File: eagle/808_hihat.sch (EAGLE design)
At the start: 127 parts, among them IC1 TL072P, IC2 TL072P, Q21* BC546, Q22* BC546, Q23* BC546, Q24* BC546, Q26* BC546, Q27* BC546, Q28* BC546, Q29* BC546, Q3* BC546, Q30* BC546, Q31* BC546, Q4* BC546, Q7* BC556, Q8* BC556, U4 4584N

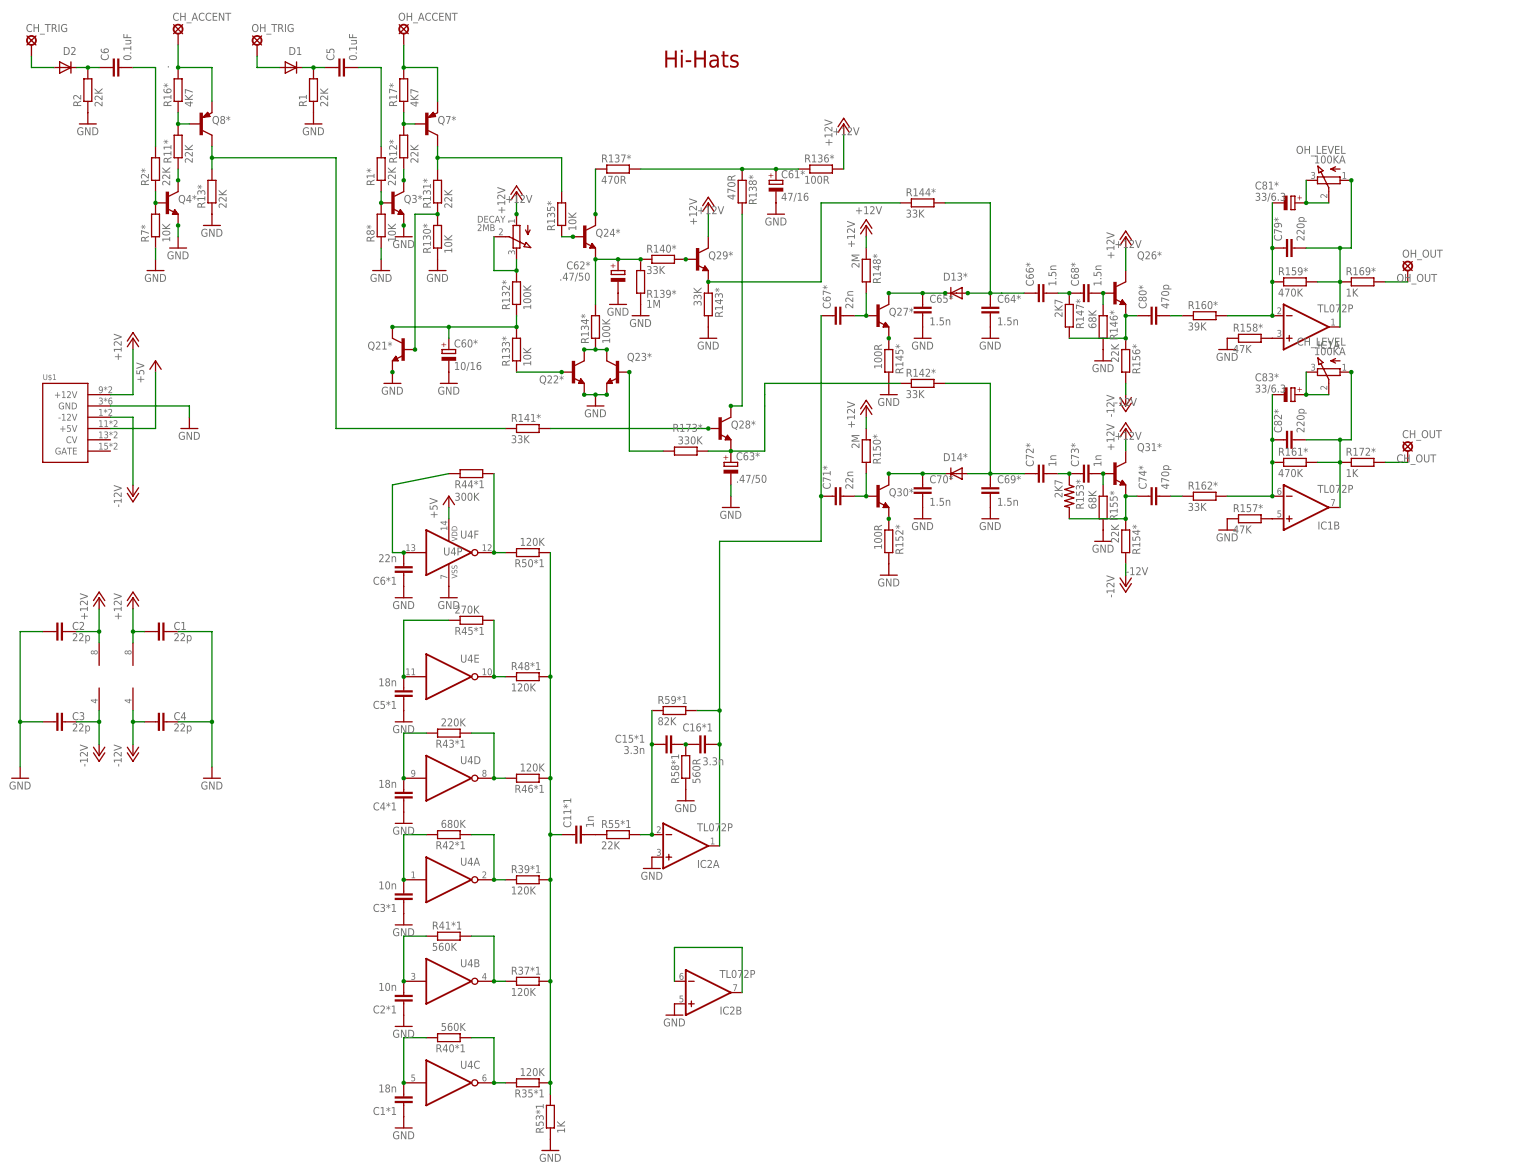
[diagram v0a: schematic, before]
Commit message: replaced parts
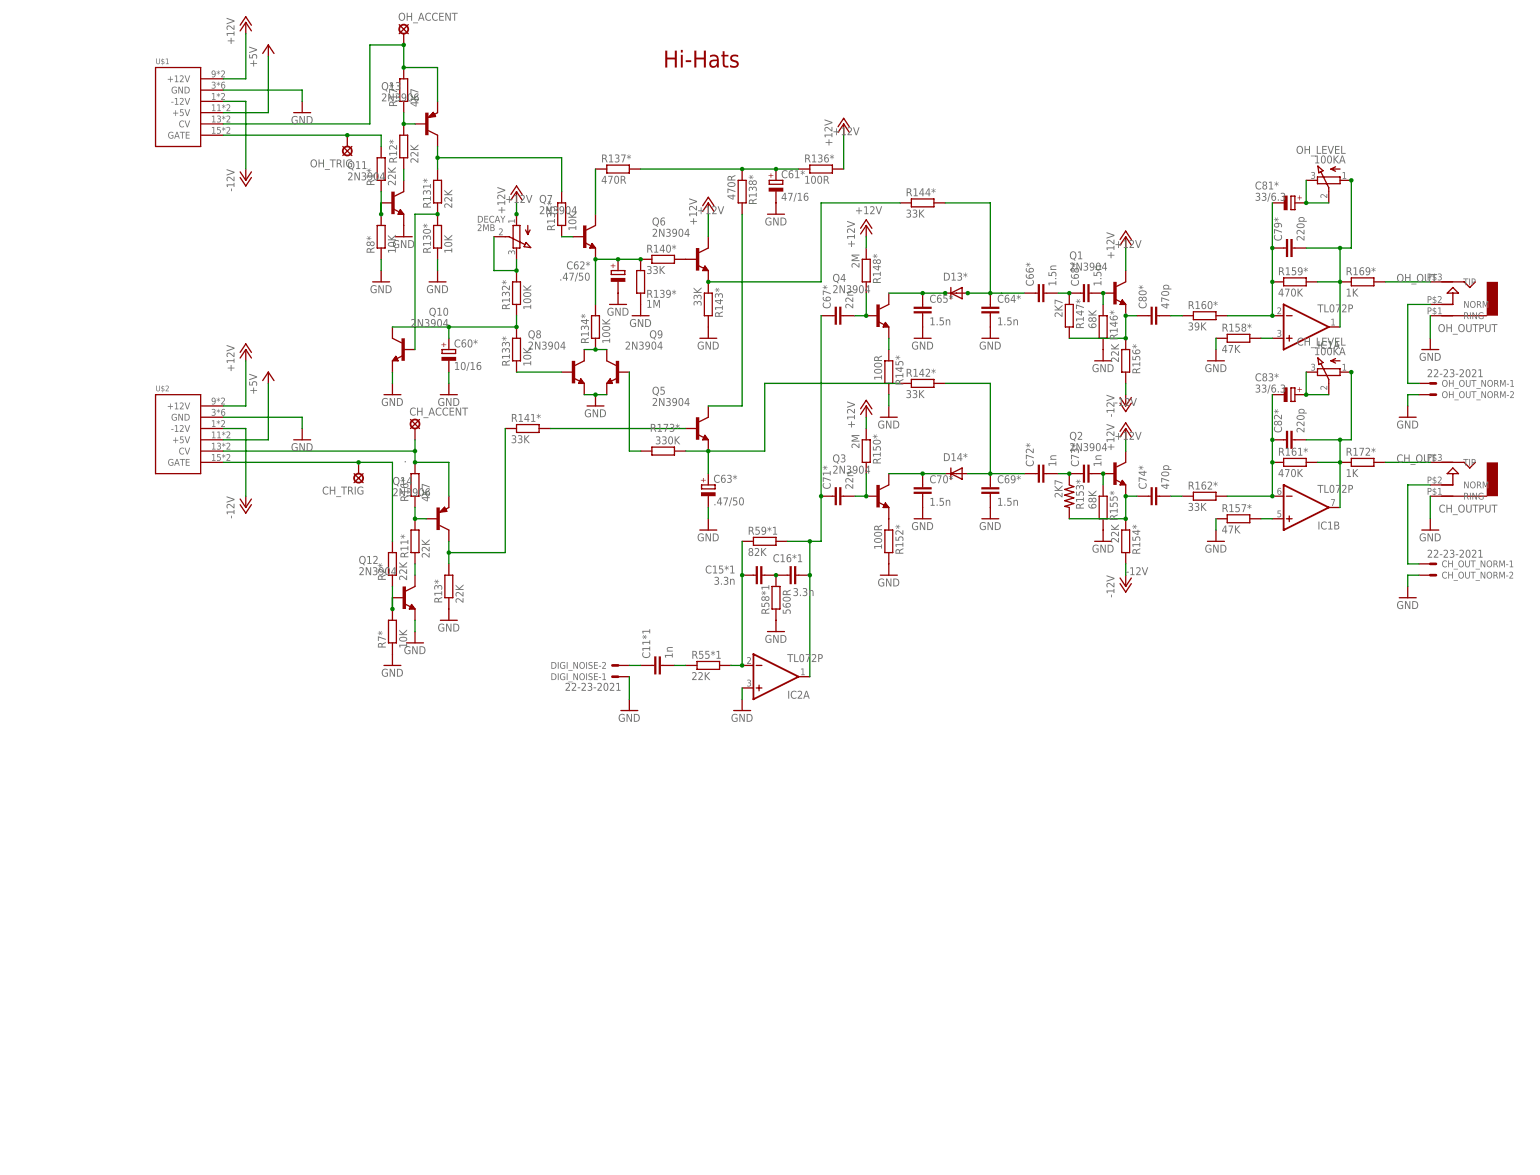
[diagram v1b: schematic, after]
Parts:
- removed C1, C2, C3, C4: 22p, TR808clone:C-EU025-025X050
- removed C1*1, C4*1, C5*1: 18n, TR808clone:C-EU4MM_PITCH
- removed C2*1, C3*1: 10n, TR808clone:C-EU3.5MM_PITCH
- removed C5, C6: 0.1uF, TR808clone:C-EU3.5MM_PITCH
- removed C6*1: 22n, TR808clone:C-EU4MM_PITCH
- removed CH_OUT, OH_OUT: LSP11, solpad:LSP11
- removed D1, D2: 1N4148DO35-7, TR808clone:1N4148DO35-7
- removed Q21*, Q22*, Q23*, Q24*, Q26*, Q27*, Q28*, Q29*, Q3*, Q30*, Q31*, Q4*: BC546, transistor:BC546-NPN-TO92-CBE
- removed Q7*, Q8*: BC556, transistor:BC556A-PNP-TO92-EBC
- removed R1, R2: 22K, TR808clone:R-EU_0207/5V
- removed R35*1, R37*1, R39*1, R46*1, R48*1, R50*1: 120K, TR808clone:R-EU_0207/5V
- removed R40*1, R41*1: 560K, TR808clone:R-EU_0207/5V
- removed R42*1: 680K, TR808clone:R-EU_0207/5V
- removed R43*1: 220K, TR808clone:R-EU_0207/5V
- removed R44*1: 300K, TR808clone:R-EU_0207/5V
- removed R45*1: 270K, TR808clone:R-EU_0207/5V
- removed R53*1: 1K, TR808clone:R-EU_0207/5V
- removed U4: 4584N, TR808clone:4584N
- added CH_OUTPUT, OH_OUTPUT: AUDIO-JACK, erthenvar:AUDIO-JACK
- added CH_OUT_NORM, DIGI_NOISE, OH_OUT_NORM: 22-23-2021, con-molex:22-23-2021
- added Q1, Q10, Q11, Q12, Q2, Q3, Q4, Q5, Q6, Q7, Q8, Q9: 2N3904, 808_lt:2N3904
- added Q13, Q14: 2N3906, 808_lt:2N3906
- added U$2: POWER, eurorack:POWER
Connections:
- removed net N$12: R35*1.2, R40*1.1, U4C.O
- removed net N$13: R37*1.1, R41*1.2, U4B.O
- removed net N$14: R43*1.1, R46*1.2, U4D.O
- removed net N$15: C5*1.2, R45*1.1, U4E.I
- removed net N$16: C6*1.2, R44*1.1, U4F.I
- removed net N$19: R39*1.1, R42*1.1, U4A.O
- removed net N$22: C5.1, D1.C, R1.2
- removed net N$23: D1.A, OH_TRIG.MP
- removed net N$24: C6.1, D2.C, R2.2
- removed net N$26: CH_TRIG.MP, D2.A
- removed net N$27: IC2B.-IN, IC2B.OUT
- removed net N$583: Q30*.E, R152*.1
- removed net N$584: Q27*.E, R145*.1
- removed net N$606: Q29*.B, R140*.2
- removed net N$9: C4*1.2, R43*1.2, U4D.I
- removed net TP1: R45*1.2, R48*1.1, U4E.O
- removed net TP2: R44*1.2, R50*1.2, U4F.O
- new net N$10: OH_OUTPUT.NORM, OH_OUT_NORM-1.S
- new net N$11: CH_OUTPUT.NORM, CH_OUT_NORM-1.S
- net +12V: now also Q1.C, Q2.C, Q6.C, U$2.+12V; no longer C1.1, C2.2, IC1P.V+, IC2P.V+, Q26*.C, Q29*.C, Q31*.C
- net +5V: now also U$2.+5V; no longer U4P.VDD
- net -12V: now also U$2.-12V; no longer C3.2, C4.1, IC1P.V-, IC2P.V-
- net .: now also Q14.E, U$2.CV; no longer Q8*.E
- net CH_OUT: now also CH_OUTPUT.TIP; no longer CH_OUT.MP
- net GND: now also CH_OUTPUT.RING, CH_OUT_NORM-2.S, DIGI_NOISE-1.S, OH_OUTPUT.RING, OH_OUT_NORM-2.S, Q10.E, Q11.E, Q12.E, Q8.E, Q9.E, U$2.GND; no longer C1*1.1, C1.2, C2*1.1, C2.1, C3*1.1, C3.1, C4*1.1, C4.2, C5*1.1, C6*1.1, IC2B.+IN, Q21*.E, Q22*.E, Q23*.E, Q3*.E, Q4*.E, R1.1, R2.1, R53*1.1, U4P.VSS
- net N$17: now also Q13.E, U$1.CV; no longer Q7*.E
- net N$18: now also OH_TRIG.MP, U$1.GATE; no longer C5.2
- net N$2: now also DIGI_NOISE-2.S; no longer R35*1.1, R37*1.2, R39*1.2, R46*1.1, R48*1.2, R50*1.1, R53*1.2
- net N$25: now also CH_TRIG.MP, U$2.GATE; no longer C6.2
- net N$559: now also Q12.B; no longer Q4*.B
- net N$560: now also Q14.B; no longer Q8*.B
- net N$562: now also Q12.C; no longer Q4*.C
- net N$563: now also Q14.C; no longer Q8*.C
- net N$566: now also Q11.B; no longer Q3*.B
- net N$567: now also Q13.B; no longer Q7*.B
- net N$568: now also Q11.C; no longer Q3*.C
- net N$569: now also Q13.C; no longer Q7*.C
- net N$571: now also Q7.C; no longer Q24*.C
- net N$572: now also Q7.B; no longer Q24*.B
- net N$573: now also Q7.E; no longer Q24*.E
- net N$574: now also Q8.C, Q9.C; no longer Q22*.C, Q23*.C
- net N$575: now also Q8.B; no longer Q22*.B
- net N$576: now also Q10.C; no longer Q21*.C
- net N$578: now also Q5.B; no longer Q28*.B
- net N$579: now also Q5.C; no longer Q28*.C
- net N$580: now also Q9.B; no longer Q23*.B
- net N$581: now also Q5.E; no longer Q28*.E
- net N$582: now also Q6.E; no longer Q29*.E
- net N$585: now also Q3.B; no longer Q30*.B
- net N$586: now also Q4.B; no longer Q27*.B
- net N$587: now also Q3.C; no longer Q30*.C
- net N$588: now also Q4.C; no longer Q27*.C
- net N$591: now also Q1.B; no longer Q26*.B
- net N$592: now also Q2.B; no longer Q31*.B
- net N$6: now also Q6.B, R140*.2; no longer C1*1.2, R40*1.2, U4C.I
- net N$604: now also Q10.B; no longer Q21*.B
- net N$607: now also Q1.E; no longer Q26*.E
- net N$608: now also Q2.E; no longer Q31*.E
- net N$7: now also Q4.E, R145*.1; no longer C2*1.2, R41*1.1, U4B.I
- net N$8: now also Q3.E, R152*.1; no longer C3*1.2, R42*1.2, U4A.I
- net OH_OUT: now also OH_OUTPUT.TIP; no longer OH_OUT.MP
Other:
- moved on the sheet: C11*1, C15*1, C16*1, C63*, CH_ACCENT, CH_TRIG, IC2A, OH_TRIG, R11*, R13*, R145*, R157*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
